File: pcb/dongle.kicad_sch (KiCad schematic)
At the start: 32 parts, among them J1 USB_A, J2 Conn_01x01_Pin, J3 Conn_01x01_Pin, J4 Conn_01x01_Pin, J5 Conn_01x01_Pin, SW1 SW_Push_45deg, U3 nRF52833_QDxx, Y1 Crystal_GND24

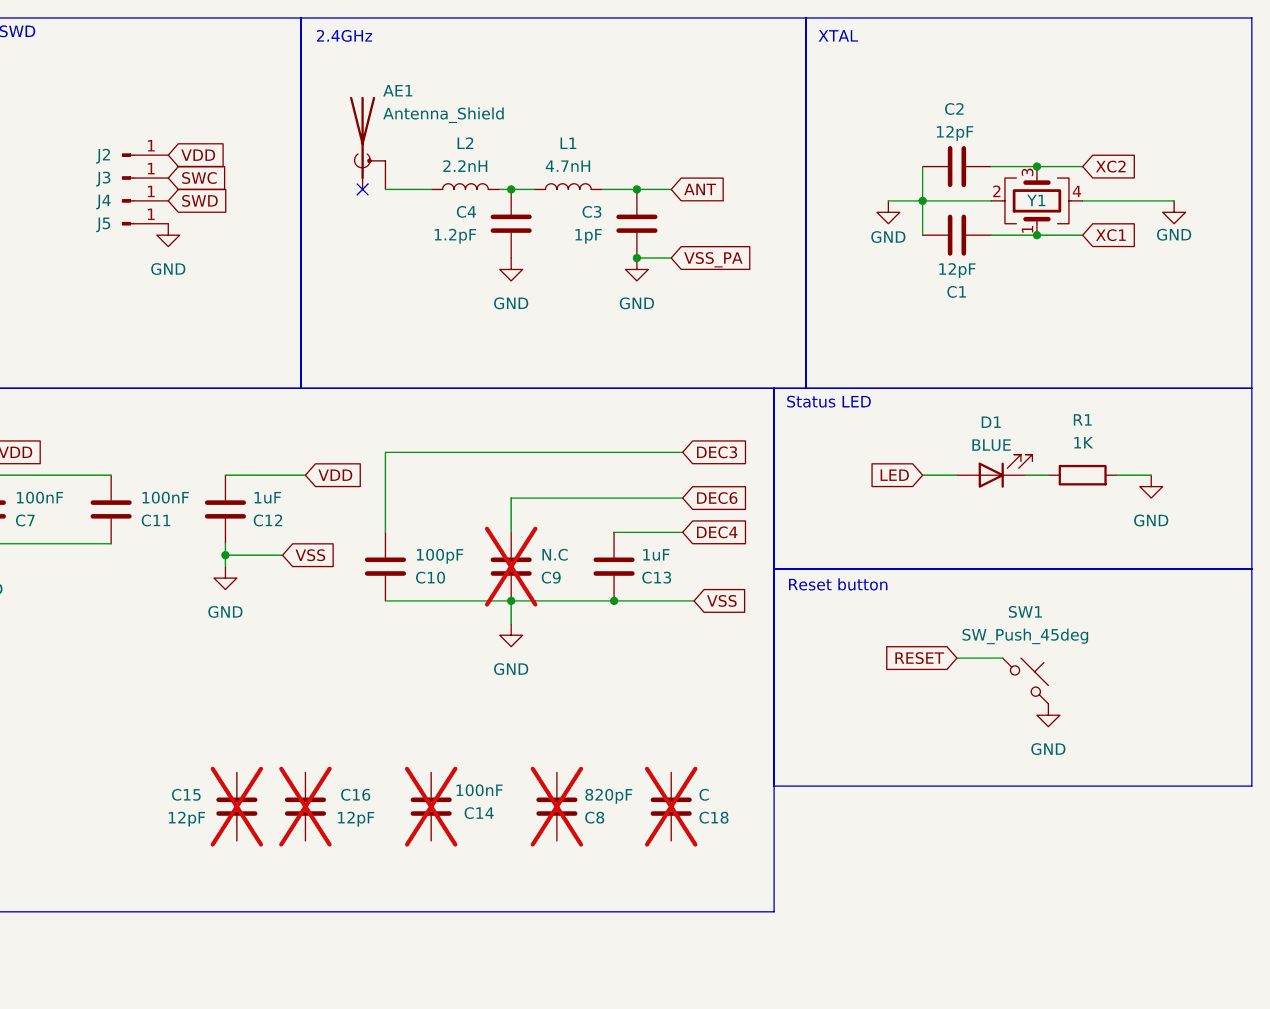
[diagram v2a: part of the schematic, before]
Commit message: udpate footprint
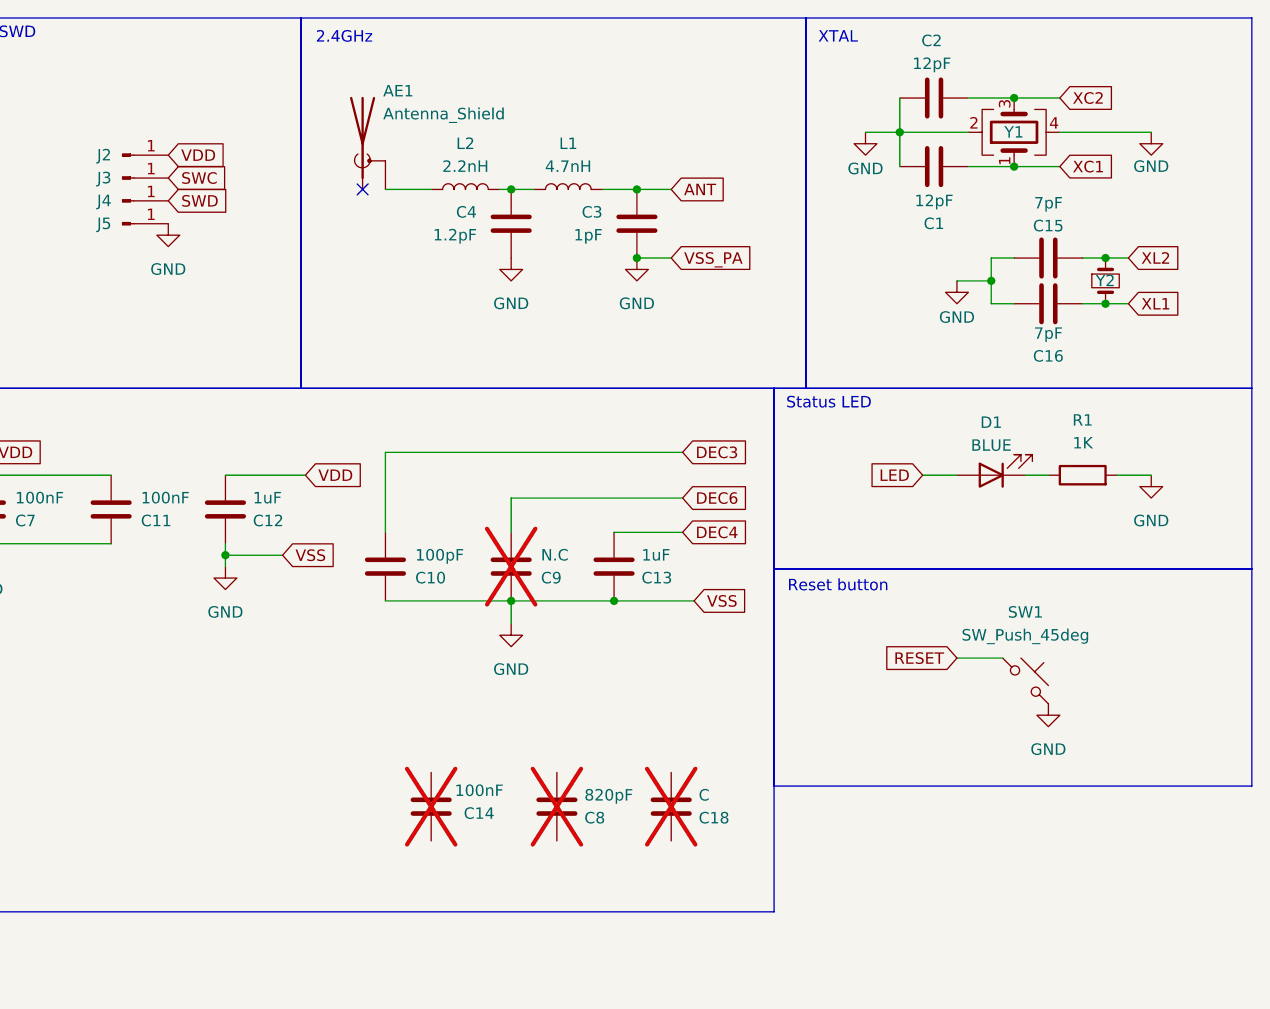
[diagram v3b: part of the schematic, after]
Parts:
- added Y2: Crystal_Small, dongle:Crystal_SMD_3215-2Pin_3.2x1.5mm, symbol dongle:Crystal_Small
- AE1: footprint dongle:ANTC5020X110N -> dongle:AN9520-245
- C15, C16: value 12pF -> 7pF; footprint dongle:C_0201_0603Metric_Pad0.64x0.40mm_HandSolder -> dongle:C_0201_0603Metric; now fitted; now in the parts list
- Y1: footprint dongle:Crystal_SMD_3225-4Pin_3.2x2.5mm -> dongle:Crystal_SMD_2520-4Pin_2.5x2.0mm
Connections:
- net GND: now also C15.2, C16.1
- net XL1: now also C16.2, Y2.2
- net XL2: now also C15.1, Y2.1
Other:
- moved on the sheet: C1, C2, Y1

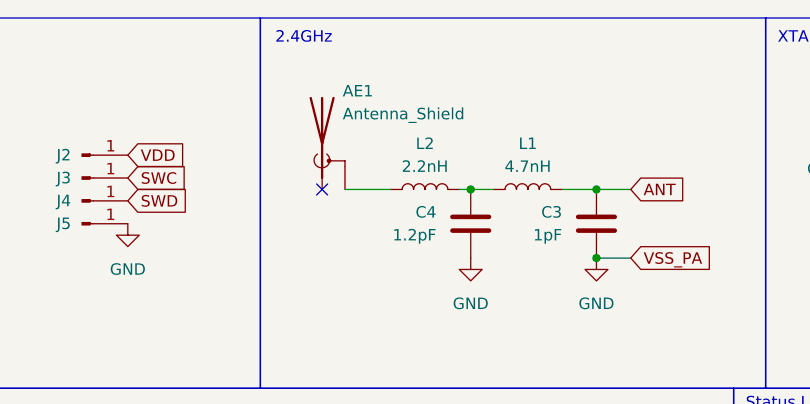
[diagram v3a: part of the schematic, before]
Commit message: upload v0.1
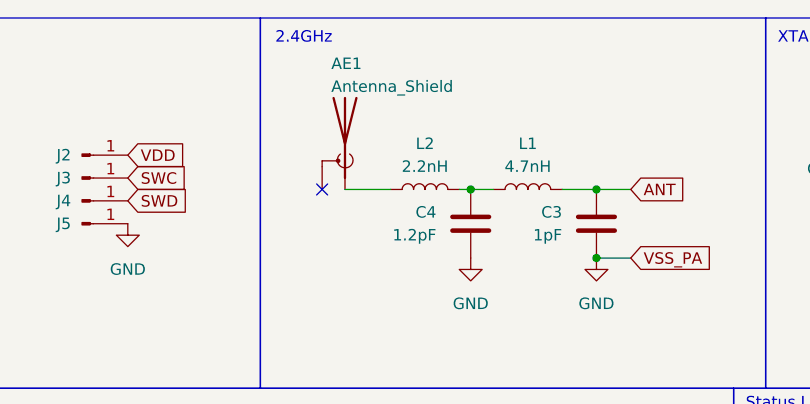
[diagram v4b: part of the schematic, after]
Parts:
- J1: footprint dongle:USB_A_Connfly_DS1098_Horizontal -> dongle:USB_A_Molex_48037-2200_Horizontal
- SW1: footprint dongle:TS342A2P -> dongle:SW_SPST_B3U-1000P
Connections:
- net at L2.2: now also AE1.1 (A); no longer AE1.2 (Shield)
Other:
- moved on the sheet: AE1
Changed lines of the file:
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@@
 	)
 	(no_connect
-		(at 92.71 71.12)
+		(at 185.42 31.75)
 	)
 	(no_connect
-		(at 185.42 31.75)
+		(at 92.71 71.12)
 	)
 	(no_connect
@@
 			)
 		)
-		(property "Footprint" "dongle:TS342A2P"
+		(property "Footprint" "dongle:SW_SPST_B3U-1000P"
 			(at 259.08 86.36 0)
 			(effects
@@
 			)
 		)
-		(property "Footprint" "dongle:USB_A_Connfly_DS1098_Horizontal"
+		(property "Footprint" "dongle:USB_A_Molex_48037-2200_Horizontal"
 			(at 127 33.02 0)
 			(effects
@@
 	(symbol
 		(lib_id "dongle:Antenna_Shield")
-		(at 185.42 26.67 0)
+		(at 187.96 26.67 0)
+		(mirror y)
 		(unit 1)
 		(exclude_from_sim no)
@@
 		(dnp no)
 		(property "Reference" "AE1"
-			(at 187.706 20.828 0)
+			(at 186.436 17.78 0)
 			(effects
 				(font
 					(size 1.27 1.27)
 				)
-				(justify left)
+				(justify right)
 			)
 		)
 		(property "Value" "Antenna_Shield"
-			(at 187.706 23.368 0)
+			(at 186.436 20.32 0)
 			(effects
 				(font
 					(size 1.27 1.27)
 				)
-				(justify left)
+				(justify right)
 			)
 		)
 		(property "Footprint" "dongle:AN9520-245"
-			(at 185.42 24.13 0)
+			(at 187.96 24.13 0)
 			(effects
 				(font
@@
 		)
 		(property "Datasheet" "~"
-			(at 185.42 24.13 0)
+			(at 187.96 24.13 0)
 			(effects
 				(font
@@
 		)
 		(property "Description" "Antenna with extra pin for shielding"
-			(at 185.42 26.67 0)
+			(at 187.96 26.67 0)
 			(effects
 				(font

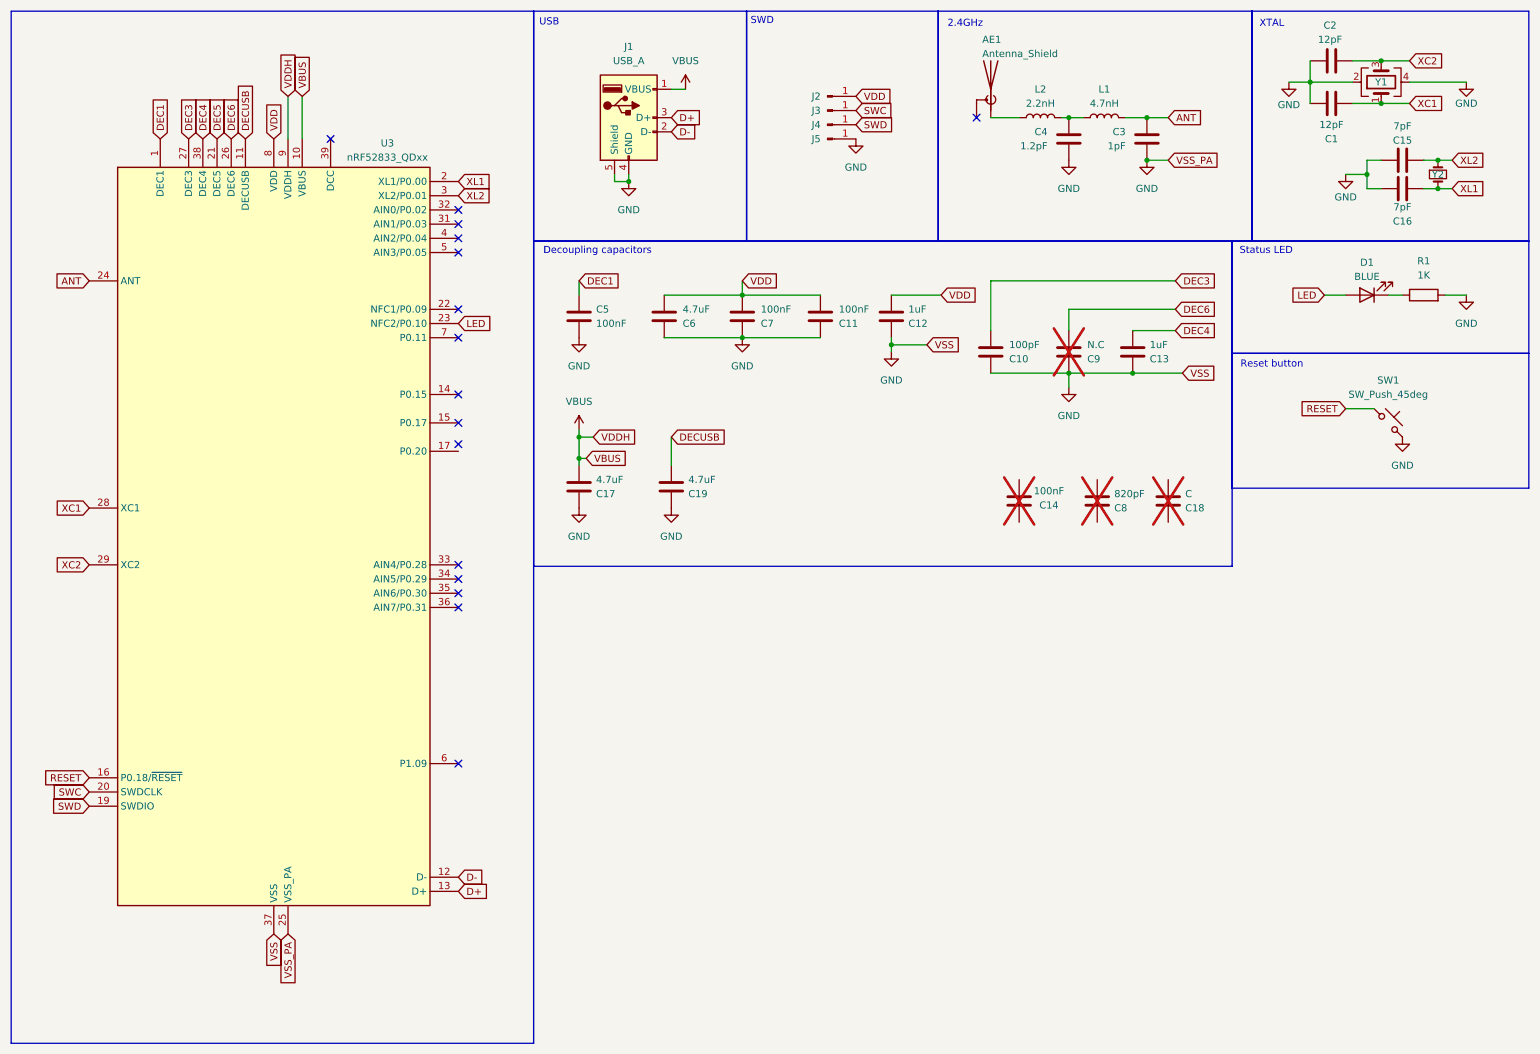
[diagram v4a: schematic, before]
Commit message: clear pcb
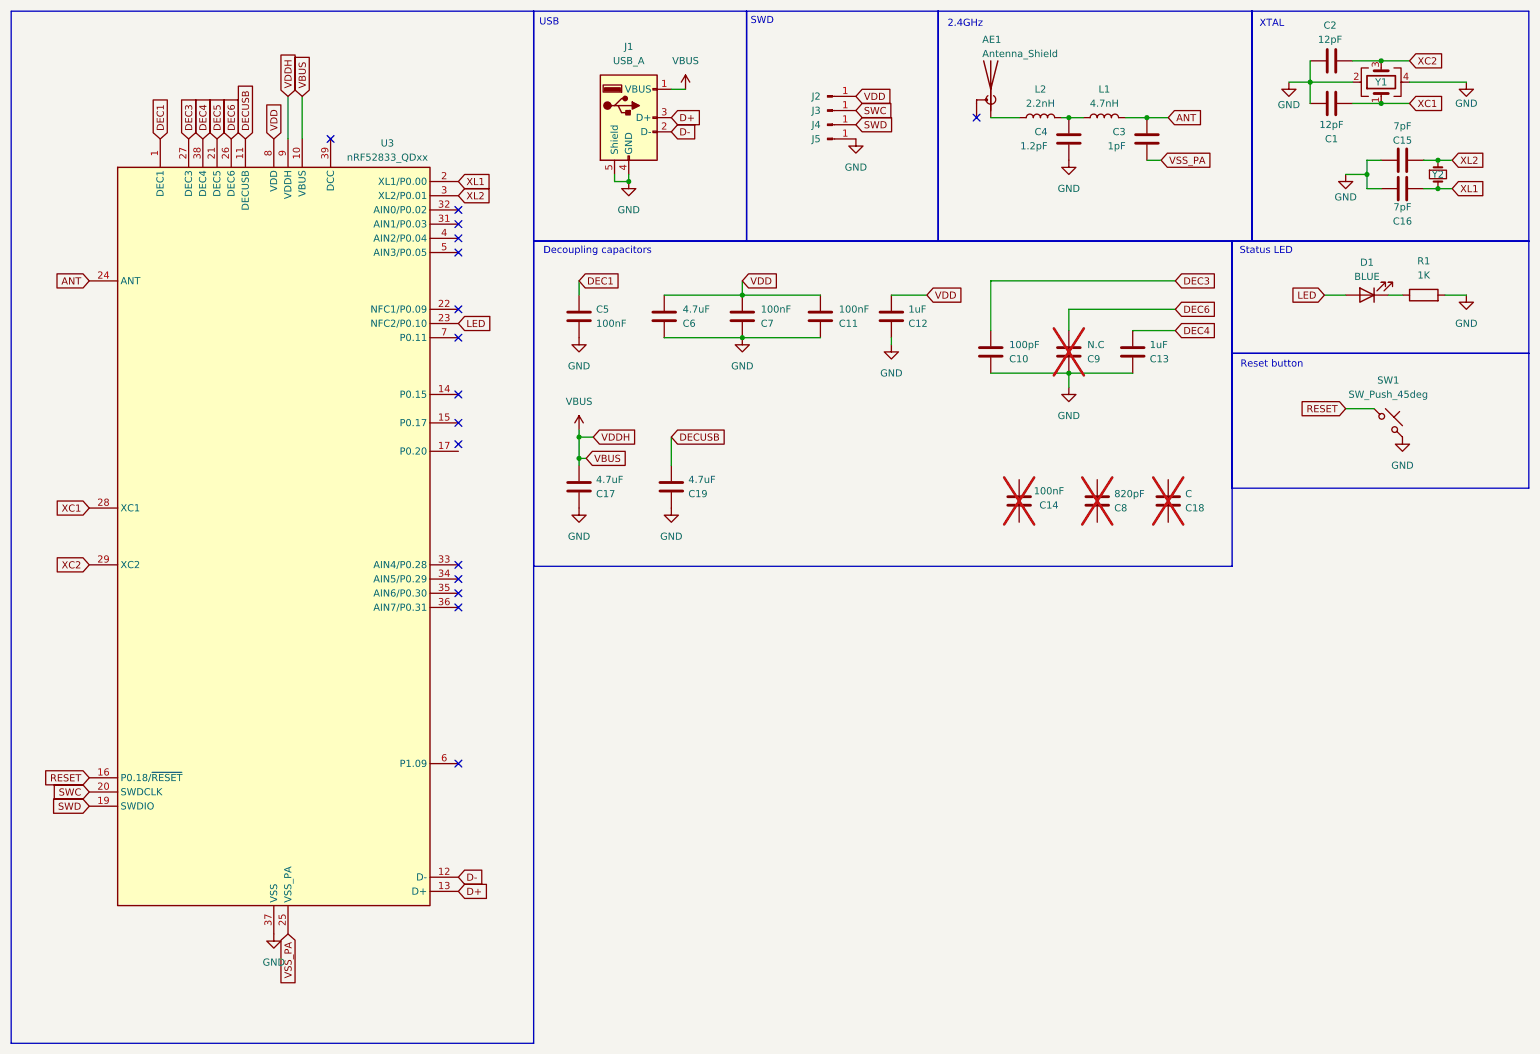
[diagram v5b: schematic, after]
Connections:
- net GND: no longer C3.1, U3.25 (VSS_PA)
- new net VSS_PA: C3.1, U3.25 (VSS_PA)
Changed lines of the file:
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@@
-	)
-	(junction
-		(at 170.18 72.39)
-		(diameter 0)
-		(color 0 0 0 0)
 	)
 	(junction
@@
 	)
 	(junction
-		(at 213.36 77.47)
-		(diameter 0)
-		(color 0 0 0 0)
-	)
-	(junction
 		(at 123.19 43.18)
 		(diameter 0)
@@
 		(color 0 0 0 0)
 	)
-	(junction
-		(at 215.9 39.37)
-		(diameter 0)
-		(color 0 0 0 0)
-	)
 	(no_connect
 		(at 92.71 147.32)
@@
 	(wire
 		(pts
-			(xy 179.07 63.5) (xy 170.18 63.5)
-		)
-		(stroke
-			(width 0)
-			(type default)
-		)
-	)
-	(wire
-		(pts
-			(xy 222.25 77.47) (xy 213.36 77.47)
+			(xy 176.53 63.5) (xy 170.18 63.5)
 		)
 		(stroke
@@
 	(wire
 		(pts
-			(xy 170.18 72.39) (xy 170.18 73.66)
+			(xy 170.18 71.12) (xy 170.18 72.39)
 		)
 		(stroke
@@
 	(wire
 		(pts
-			(xy 170.18 71.12) (xy 170.18 72.39)
-		)
-		(stroke
-			(width 0)
-			(type default)
-		)
-	)
-	(wire
-		(pts
-			(xy 219.71 39.37) (xy 215.9 39.37)
+			(xy 218.44 39.37) (xy 215.9 39.37)
 		)
 		(stroke
@@
 	(wire
 		(pts
-			(xy 176.53 72.39) (xy 170.18 72.39)
-		)
-		(stroke
-			(width 0)
-			(type default)
-		)
-	)
-	(wire
-		(pts
 			(xy 251.46 63.5) (xy 247.65 63.5)
 		)
@@
 		)
 	)
-	(global_label "VSS"
-		(shape input)
-		(at 176.53 72.39 0)
-		(fields_autoplaced yes)
-		(effects
-			(font
-				(size 1.27 1.27)
-			)
-			(justify left)
-		)
-		(property "Intersheetrefs" "${INTERSHEET_REFS}"
-			(at 183.0228 72.39 0)
-			(effects
-				(font
-					(size 1.27 1.27)
-				)
-				(justify left)
-				(hide yes)
-			)
-		)
-	)
 	(global_label "VDD"
 		(shape input)
-		(at 179.07 63.5 0)
-		(fields_autoplaced yes)
-		(effects
-			(font
-				(size 1.27 1.27)
-			)
-			(justify left)
-		)
-		(property "Intersheetrefs" "${INTERSHEET_REFS}"
-			(at 185.6838 63.5 0)
+		(at 176.53 63.5 0)
+		(fields_autoplaced yes)
+		(effects
+			(font
+				(size 1.27 1.27)
+			)
+			(justify left)
+		)
+		(property "Intersheetrefs" "${INTERSHEET_REFS}"
+			(at 183.1438 63.5 0)
 			(effects
 				(font
@@
 		)
 	)
-	(global_label "VSS"
-		(shape input)
-		(at 222.25 77.47 0)
-		(fields_autoplaced yes)
-		(effects
-			(font
-				(size 1.27 1.27)
-			)
-			(justify left)
-		)
-		(property "Intersheetrefs" "${INTERSHEET_REFS}"
-			(at 228.7428 77.47 0)
-			(effects
-				(font
-					(size 1.27 1.27)
-				)
-				(justify left)
-				(hide yes)
-			)
-		)
-	)
 	(global_label "VBUS"
 		(shape input)
@@
 	(global_label "VSS_PA"
 		(shape input)
-		(at 219.71 39.37 0)
-		(fields_autoplaced yes)
-		(effects
-			(font
-				(size 1.27 1.27)
-			)
-			(justify left)
-		)
-		(property "Intersheetrefs" "${INTERSHEET_REFS}"
-			(at 229.529 39.37 0)
+		(at 218.44 39.37 0)
+		(fields_autoplaced yes)
+		(effects
+			(font
+				(size 1.27 1.27)
+			)
+			(justify left)
+		)
+		(property "Intersheetrefs" "${INTERSHEET_REFS}"
+			(at 228.259 39.37 0)
 			(effects
 				(font
@@
 				)
 				(justify left)
-				(hide yes)
-			)
-		)
-	)
-	(global_label "VSS"
-		(shape input)
-		(at 59.69 177.8 270)
-		(fields_autoplaced yes)
-		(effects
-			(font
-				(size 1.27 1.27)
-			)
-			(justify right)
-		)
-		(property "Intersheetrefs" "${INTERSHEET_REFS}"
-			(at 59.69 184.2928 90)
-			(effects
-				(font
-					(size 1.27 1.27)
-				)
-				(justify right)
 				(hide yes)
 			)
@@
 				(path "/81b8789c-509b-48aa-aabd-6327c54a25df"
 					(reference "J5")
-					(unit 1)
-				)
-			)
-		)
-	)
-	(symbol
-		(lib_id "PNCATEHO_lowair:GND")
-		(at 215.9 39.37 0)
-		(mirror y)
-		(unit 1)
-		(exclude_from_sim no)
-		(in_bom yes)
-		(on_board yes)
-		(dnp no)
-		(fields_autoplaced yes)
-		(property "Reference" "#PWR028"
-			(at 215.9 45.72 0)
-			(effects
-				(font
-					(size 1.27 1.27)
-				)
-				(hide yes)
-			)
-		)
-		(property "Value" "GND"
-			(at 215.9 44.45 0)
-			(effects
-				(font
-					(size 1.27 1.27)
-				)
-			)
-		)
-		(property "Footprint" ""
-			(at 215.9 39.37 0)
-			(effects
-				(font
-					(size 1.27 1.27)
-				)
-				(hide yes)
-			)
-		)
-		(property "Datasheet" ""
-			(at 215.9 39.37 0)
-			(effects
-				(font
-					(size 1.27 1.27)
-				)
-				(hide yes)
-			)
-		)
-		(property "Description" "Power symbol creates a global label with name \"GND\" , ground"
-			(at 215.9 39.37 0)
-			(effects
-				(font
-					(size 1.27 1.27)
-				)
-				(hide yes)
-			)
-		)
-		(pin "1"
-		)
-		(instances
-			(project "PNCATEHO_lowair"
-				(path "/81b8789c-509b-48aa-aabd-6327c54a25df"
-					(reference "#PWR028")
 					(unit 1)
 				)
@@
 	)
 	(symbol
+		(lib_id "Library:GND")
+		(at 59.69 177.8 0)
+		(unit 1)
+		(exclude_from_sim no)
+		(in_bom yes)
+		(on_board yes)
+		(dnp no)
+		(fields_autoplaced yes)
+		(property "Reference" "#PWR015"
+			(at 59.69 184.15 0)
+			(effects
+				(font
+					(size 1.27 1.27)
+				)
+				(hide yes)
+			)
+		)
+		(property "Value" "GND"
+			(at 59.69 182.88 0)
+			(effects
+				(font
+					(size 1.27 1.27)
+				)
+			)
+		)
+		(property "Footprint" ""
+			(at 59.69 177.8 0)
+			(effects
+				(font
+					(size 1.27 1.27)
+				)
+				(hide yes)
+			)
+		)
+		(property "Datasheet" ""
+			(at 59.69 177.8 0)
+			(effects
+				(font
+					(size 1.27 1.27)
+				)
+				(hide yes)
+			)
+		)
+		(property "Description" "Global ground symbol"
+			(at 59.69 187.198 0)
+			(effects
+				(font
+					(size 1.27 1.27)
+				)
+				(hide yes)
+			)
+		)
+		(pin "1"
+		)
+		(instances
+			(project "dongle"
+				(path "/81b8789c-509b-48aa-aabd-6327c54a25df"
+					(reference "#PWR015")
+					(unit 1)
+				)
+			)
+		)
+	)
+	(symbol
 		(lib_id "dongle:SW_Push_45deg")
 		(at 259.08 86.36 0)
@@
 	(symbol
 		(lib_id "Library:GND")
-		(at 170.18 73.66 0)
+		(at 170.18 72.39 0)
 		(unit 1)
 		(exclude_from_sim no)
@@
 		(fields_autoplaced yes)
 		(property "Reference" "#PWR07"
-			(at 170.18 80.01 0)
+			(at 170.18 78.74 0)
 			(effects
 				(font
@@
 		)
 		(property "Value" "GND"
-			(at 170.18 78.74 0)
+			(at 170.18 77.47 0)
 			(effects
 				(font
@@
 		)
 		(property "Footprint" ""
-			(at 170.18 73.66 0)
+			(at 170.18 72.39 0)
 			(effects
 				(font
@@
 		)
 		(property "Datasheet" ""
-			(at 170.18 73.66 0)
+			(at 170.18 72.39 0)
 			(effects
 				(font
@@
 		)
 		(property "Description" "Global ground symbol"
-			(at 170.18 83.058 0)
-			(effects
-				(font
+			(at 170.18 81.788 0)
+			(effects
+				(font
